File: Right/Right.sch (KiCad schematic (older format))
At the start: 105 parts, among them SW1 SW_PUSH, SW10 SW_PUSH, SW100 SW_Push_Dual_R, SW101 SW_Push_Dual_R, SW102 SW_Push_Dual_R, SW11 SW_PUSH, SW12 SW_PUSH, SW13 SW_PUSH, SW14 SW_PUSH, SW15 SW_PUSH, SW16 SW_PUSH, SW17 SW_PUSH, SW18 SW_PUSH, SW19 SW_PUSH, SW2 SW_PUSH, SW20 SW_PUSH, SW200 SW_SPDT, SW21 SW_PUSH, SW22 SW_PUSH, SW23 SW_PUSH, SW24 SW_PUSH, SW25 SW_PUSH, SW26 SW_PUSH, SW27 SW_PUSH, SW28 SW_PUSH, SW29 SW_PUSH, SW3 SW_PUSH, SW30 SW_PUSH, SW31 SW_PUSH, SW32 SW_PUSH, SW33 SW_PUSH, SW34 SW_PUSH, SW35 SW_PUSH, SW36 SW_PUSH, SW37 SW_PUSH, SW38 SW_PUSH, SW39 SW_PUSH, SW4 SW_PUSH, SW40 SW_PUSH, SW41 SW_PUSH, SW42 SW_PUSH, SW43 SW_PUSH, SW44 SW_PUSH, SW45 SW_PUSH, SW5 SW_PUSH, SW6 SW_PUSH, SW7 SW_PUSH, SW8 SW_PUSH, SW9 SW_PUSH, U1 CH25-2032LF, U2 CH25-2032LF

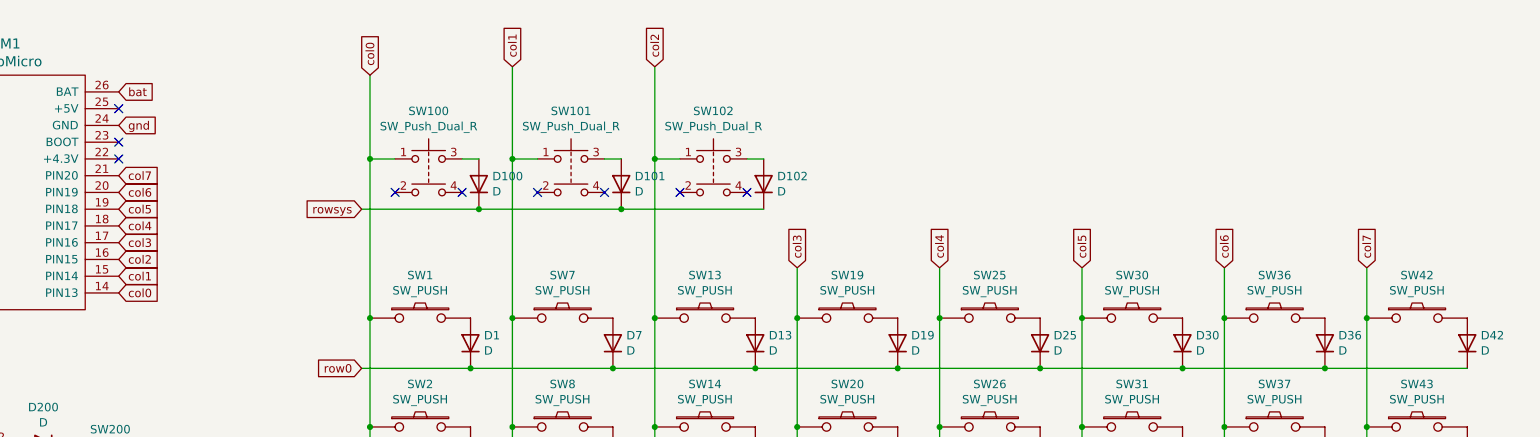
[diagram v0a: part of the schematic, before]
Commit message: 小さく
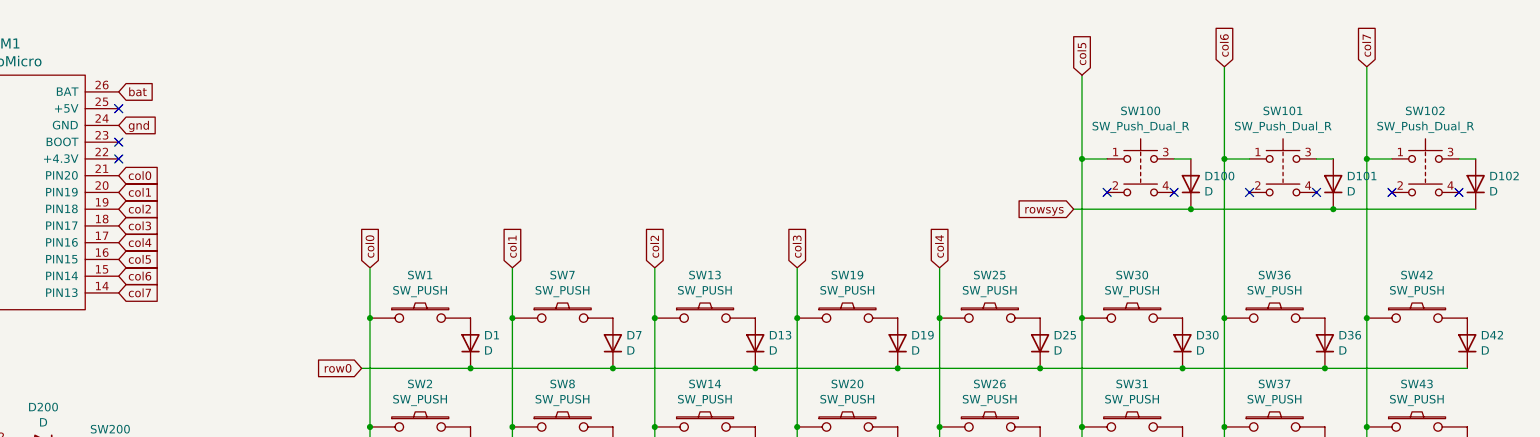
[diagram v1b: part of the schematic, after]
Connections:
- net col0: now also BPM1.21 (PIN20); no longer BPM1.14 (PIN13), SW100.1
- net col1: now also BPM1.20 (PIN19); no longer BPM1.15 (PIN14), SW101.1
- net col2: now also BPM1.19 (PIN18); no longer BPM1.16 (PIN15), SW102.1
- net col3: now also BPM1.18 (PIN17); no longer BPM1.17 (PIN16)
- net col4: now also BPM1.17 (PIN16); no longer BPM1.18 (PIN17)
- net col5: now also BPM1.16 (PIN15), SW100.1; no longer BPM1.19 (PIN18)
- net col6: now also BPM1.15 (PIN14), SW101.1; no longer BPM1.20 (PIN19)
- net col7: now also BPM1.14 (PIN13), SW102.1; no longer BPM1.21 (PIN20)
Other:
- moved on the sheet: D100, D101, D102, SW100, SW101, SW102
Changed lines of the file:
@@
 $EndComp
 Wire Wire Line
-	5750 1200 5750 1750
+	10000 1200 10000 1750
 Connection ~ 5750 2700
 Connection ~ 6350 3000
@@
 	0    -1   -1   0
 $EndComp
-Wire Wire Line
-	8300 2400 8300 2700
 Connection ~ 8300 2700
 Connection ~ 8900 3000
@@
 	0    -1   -1   0
 $EndComp
-Wire Wire Line
-	9150 2400 9150 2700
 Connection ~ 9150 2700
 Connection ~ 9750 3000
@@
 	0    -1   -1   0
 $EndComp
-Wire Wire Line
-	10000 2400 10000 2700
 Connection ~ 10000 2700
 Wire Wire Line
@@
 Text GLabel 4000 6250 0    50   Input ~ 0
 row5
-Text GLabel 4050 1250 1    50   Input ~ 0
+Text GLabel 4050 2400 1    50   Input ~ 0
 col0
-Text GLabel 4900 1200 1    50   Input ~ 0
+Text GLabel 4900 2400 1    50   Input ~ 0
 col1
-Text GLabel 5750 1200 1    50   Input ~ 0
+Text GLabel 5750 2400 1    50   Input ~ 0
 col2
 Text GLabel 6600 2400 1    50   Input ~ 0
@@
 Text GLabel 7450 2400 1    50   Input ~ 0
 col4
-Text GLabel 8300 2400 1    50   Input ~ 0
+Text GLabel 8300 1250 1    50   Input ~ 0
 col5
-Text GLabel 9150 2400 1    50   Input ~ 0
+Text GLabel 9150 1200 1    50   Input ~ 0
 col6
-Text GLabel 10000 2400 1    50   Input ~ 0
+Text GLabel 10000 1200 1    50   Input ~ 0
 col7
 $Comp
@@
 Text GLabel 1150 1850 0    50   Input ~ 0
 row5
-Text GLabel 2550 2550 2    50   Input ~ 0
-col0
-Text GLabel 2550 2450 2    50   Input ~ 0
-col1
-Text GLabel 2550 2350 2    50   Input ~ 0
-col2
-Text GLabel 2550 2250 2    50   Input ~ 0
-col3
-Text GLabel 2550 2150 2    50   Input ~ 0
-col4
-Text GLabel 2550 2050 2    50   Input ~ 0
-col5
-Text GLabel 2550 1950 2    50   Input ~ 0
-col6
-Text GLabel 2550 1850 2    50   Input ~ 0
-col7
 $Comp
 L CH25-2032LF:CH25-2032LF U1
@@
 	1100 3900 1100 3650
 NoConn ~ 2700 3750
-NoConn ~ 4200 1950
-NoConn ~ 4600 1950
+NoConn ~ 8450 1950
+NoConn ~ 8850 1950
 $Comp
 L Device:D D100
 U 1 1 5F386B99
-P 4700 1900
-F 0 "D100" V 4746 1820 50  0000 R CNN
-F 1 "D" V 4655 1820 50  0000 R CNN
-F 2 "Diode_THT:D_DO-35_SOD27_P7.62mm_Horizontal" H 4700 1900 50  0001 C CNN
-F 3 "~" H 4700 1900 50  0001 C CNN
-	1    4700 1900
-	0    -1   -1   0
-$EndComp
-Wire Wire Line
-	4600 1750 4700 1750
-Wire Wire Line
-	4700 2050 4000 2050
-Text GLabel 4000 2050 0    50   Input ~ 0
+P 8950 1900
+F 0 "D100" V 8996 1820 50  0000 R CNN
+F 1 "D" V 8905 1820 50  0000 R CNN
+F 2 "Diode_THT:D_DO-35_SOD27_P7.62mm_Horizontal" H 8950 1900 50  0001 C CNN
+F 3 "~" H 8950 1900 50  0001 C CNN
+	1    8950 1900
+	0    -1   -1   0
+$EndComp
+Wire Wire Line
+	8850 1750 8950 1750
+Wire Wire Line
+	8950 2050 8250 2050
+Text GLabel 8250 2050 0    50   Input ~ 0
 rowsys
 Wire Wire Line
-	4700 2050 5550 2050
-Connection ~ 4700 2050
-Wire Wire Line
-	4050 1250 4050 1750
-Wire Wire Line
-	4200 1750 4050 1750
-Connection ~ 4050 1750
-Wire Wire Line
-	4050 1750 4050 2700
-Wire Wire Line
-	4900 1200 4900 1750
-NoConn ~ 5050 1950
-NoConn ~ 5450 1950
+	8950 2050 9800 2050
+Connection ~ 8950 2050
+Wire Wire Line
+	8300 1250 8300 1750
+Wire Wire Line
+	8450 1750 8300 1750
+Connection ~ 8300 1750
+Wire Wire Line
+	9150 1200 9150 1750
+NoConn ~ 9300 1950
+NoConn ~ 9700 1950
 $Comp
 L Device:D D101
 U 1 1 5F3CEA11
-P 5550 1900
-F 0 "D101" V 5596 1820 50  0000 R CNN
-F 1 "D" V 5505 1820 50  0000 R CNN
-F 2 "Diode_THT:D_DO-35_SOD27_P7.62mm_Horizontal" H 5550 1900 50  0001 C CNN
-F 3 "~" H 5550 1900 50  0001 C CNN
-	1    5550 1900
-	0    -1   -1   0
-$EndComp
-Wire Wire Line
-	5450 1750 5550 1750
-Wire Wire Line
-	5050 1750 4900 1750
-Connection ~ 5550 2050
-Connection ~ 4900 1750
-Wire Wire Line
-	4900 1750 4900 2700
-NoConn ~ 5900 1950
-NoConn ~ 6300 1950
+P 9800 1900
+F 0 "D101" V 9846 1820 50  0000 R CNN
+F 1 "D" V 9755 1820 50  0000 R CNN
+F 2 "Diode_THT:D_DO-35_SOD27_P7.62mm_Horizontal" H 9800 1900 50  0001 C CNN
+F 3 "~" H 9800 1900 50  0001 C CNN
+	1    9800 1900
+	0    -1   -1   0
+$EndComp
+Wire Wire Line
+	9700 1750 9800 1750
+Wire Wire Line
+	9300 1750 9150 1750
+Connection ~ 9800 2050
+Connection ~ 9150 1750
+NoConn ~ 10150 1950
+NoConn ~ 10550 1950
 $Comp
 L Device:D D102
 U 1 1 5F3D4407
-P 6400 1900
-F 0 "D102" V 6446 1820 50  0000 R CNN
-F 1 "D" V 6355 1820 50  0000 R CNN
-F 2 "Diode_THT:D_DO-35_SOD27_P7.62mm_Horizontal" H 6400 1900 50  0001 C CNN
-F 3 "~" H 6400 1900 50  0001 C CNN
-	1    6400 1900
-	0    -1   -1   0
-$EndComp
-Wire Wire Line
-	6300 1750 6400 1750
-Wire Wire Line
-	5900 1750 5750 1750
-Connection ~ 5750 1750
-Wire Wire Line
-	5750 1750 5750 2700
-Wire Wire Line
-	5550 2050 6400 2050
+P 10650 1900
+F 0 "D102" V 10696 1820 50  0000 R CNN
+F 1 "D" V 10605 1820 50  0000 R CNN
+F 2 "Diode_THT:D_DO-35_SOD27_P7.62mm_Horizontal" H 10650 1900 50  0001 C CNN
+F 3 "~" H 10650 1900 50  0001 C CNN
+	1    10650 1900
+	0    -1   -1   0
+$EndComp
+Wire Wire Line
+	10550 1750 10650 1750
+Wire Wire Line
+	10150 1750 10000 1750
+Connection ~ 10000 1750
+Wire Wire Line
+	9800 2050 10650 2050
 Text GLabel 1150 2550 0    50   Input ~ 0
 rowsys
@@
 L My_Library:SW_Push_Dual_R SW102
 U 1 1 5F449060
-P 6100 1750
-F 0 "SW102" H 6100 2035 50  0000 C CNN
-F 1 "SW_Push_Dual_R" H 6100 1944 50  0000 C CNN
-F 2 "Button_Switch_THT:SW_TH_Tactile_Omron_B3F-10xx" H 6100 1950 50  0001 C CNN
-F 3 "" H 6100 1950 50  0001 C CNN
-	1    6100 1750
+P 10350 1750
+F 0 "SW102" H 10350 2035 50  0000 C CNN
+F 1 "SW_Push_Dual_R" H 10350 1944 50  0000 C CNN
+F 2 "Button_Switch_THT:SW_TH_Tactile_Omron_B3F-10xx" H 10350 1950 50  0001 C CNN
+F 3 "" H 10350 1950 50  0001 C CNN
+	1    10350 1750
 	1    0    0    -1
 $EndComp
@@
 L My_Library:SW_Push_Dual_R SW101
 U 1 1 5F44E520
-P 5250 1750
-F 0 "SW101" H 5250 2035 50  0000 C CNN
-F 1 "SW_Push_Dual_R" H 5250 1944 50  0000 C CNN
-F 2 "Button_Switch_THT:SW_TH_Tactile_Omron_B3F-10xx" H 5250 1950 50  0001 C CNN
-F 3 "" H 5250 1950 50  0001 C CNN
-	1    5250 1750
+P 9500 1750
+F 0 "SW101" H 9500 2035 50  0000 C CNN
+F 1 "SW_Push_Dual_R" H 9500 1944 50  0000 C CNN
+F 2 "Button_Switch_THT:SW_TH_Tactile_Omron_B3F-10xx" H 9500 1950 50  0001 C CNN
+F 3 "" H 9500 1950 50  0001 C CNN
+	1    9500 1750
 	1    0    0    -1
 $EndComp
@@
 L My_Library:SW_Push_Dual_R SW100
 U 1 1 5F44F80F
-P 4400 1750
-F 0 "SW100" H 4400 2035 50  0000 C CNN
-F 1 "SW_Push_Dual_R" H 4400 1944 50  0000 C CNN
-F 2 "Button_Switch_THT:SW_TH_Tactile_Omron_B3F-10xx" H 4400 1950 50  0001 C CNN
-F 3 "" H 4400 1950 50  0001 C CNN
-	1    4400 1750
-	1    0    0    -1
-$EndComp
+P 8650 1750
+F 0 "SW100" H 8650 2035 50  0000 C CNN
+F 1 "SW_Push_Dual_R" H 8650 1944 50  0000 C CNN
+F 2 "Button_Switch_THT:SW_TH_Tactile_Omron_B3F-10xx" H 8650 1950 50  0001 C CNN
+F 3 "" H 8650 1950 50  0001 C CNN
+	1    8650 1750
+	1    0    0    -1
+$EndComp
+Wire Wire Line
+	5750 2400 5750 2700
+Wire Wire Line
+	4900 2400 4900 2700
+Wire Wire Line
+	4050 2400 4050 2700
+Wire Wire Line
+	8300 1750 8300 2700
+Wire Wire Line
+	9150 1750 9150 2700
+Wire Wire Line
+	10000 1750 10000 2700
+Text GLabel 2550 2550 2    50   Input ~ 0
+col7
+Text GLabel 2550 2450 2    50   Input ~ 0
+col6
+Text GLabel 2550 2350 2    50   Input ~ 0
+col5
+Text GLabel 2550 2250 2    50   Input ~ 0
+col4
+Text GLabel 2550 2150 2    50   Input ~ 0
+col3
+Text GLabel 2550 2050 2    50   Input ~ 0
+col2
+Text GLabel 2550 1950 2    50   Input ~ 0
+col1
+Text GLabel 2550 1850 2    50   Input ~ 0
+col0
 $EndSCHEMATC

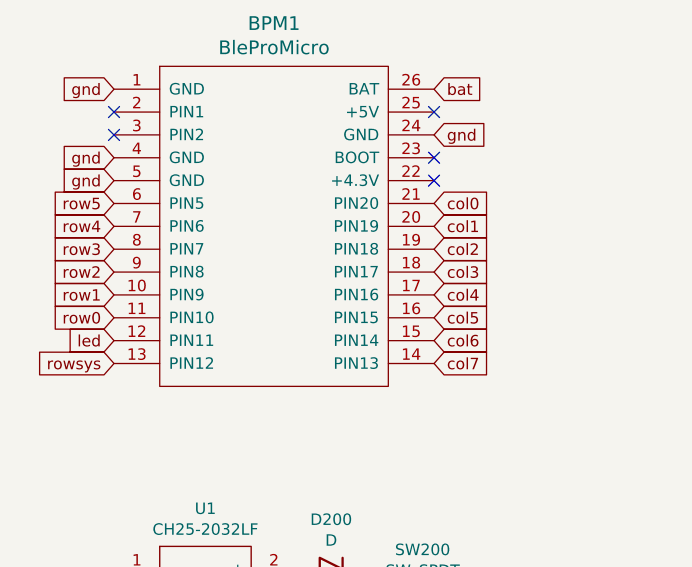
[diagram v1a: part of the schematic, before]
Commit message: 位置調整
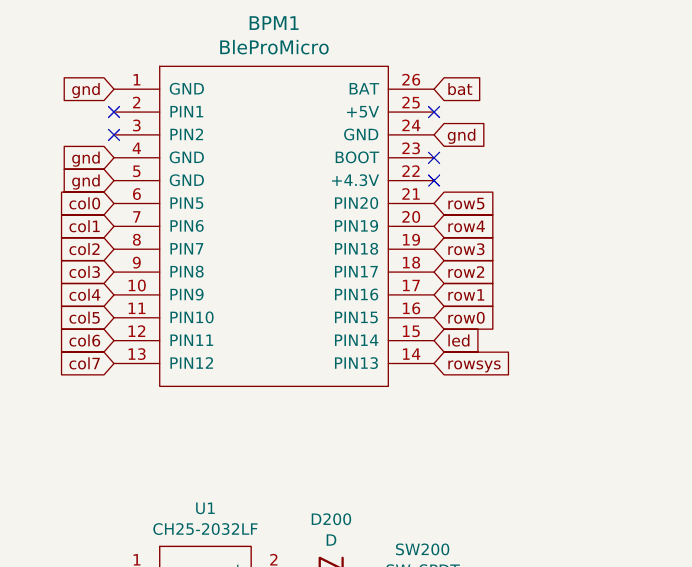
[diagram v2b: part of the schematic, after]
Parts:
- BPM1: footprint mylibrary:BLEMicroPro_reversed -> mylibrary:BLEMicroPro
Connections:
- net col0: now also BPM1.6 (PIN5); no longer BPM1.21 (PIN20)
- net col1: now also BPM1.7 (PIN6); no longer BPM1.20 (PIN19)
- net col2: now also BPM1.8 (PIN7); no longer BPM1.19 (PIN18)
- net col3: now also BPM1.9 (PIN8); no longer BPM1.18 (PIN17)
- net col4: now also BPM1.10 (PIN9); no longer BPM1.17 (PIN16)
- net col5: now also BPM1.11 (PIN10); no longer BPM1.16 (PIN15)
- net col6: now also BPM1.12 (PIN11); no longer BPM1.15 (PIN14)
- net col7: now also BPM1.13 (PIN12); no longer BPM1.14 (PIN13)
- net led: now also BPM1.15 (PIN14); no longer BPM1.12 (PIN11)
- net row0: now also BPM1.16 (PIN15); no longer BPM1.11 (PIN10)
- net row1: now also BPM1.17 (PIN16); no longer BPM1.10 (PIN9)
- net row2: now also BPM1.18 (PIN17); no longer BPM1.9 (PIN8)
- net row3: now also BPM1.19 (PIN18); no longer BPM1.8 (PIN7)
- net row4: now also BPM1.20 (PIN19); no longer BPM1.7 (PIN6)
- net row5: now also BPM1.21 (PIN20); no longer BPM1.6 (PIN5)
- net rowsys: now also BPM1.14 (PIN13); no longer BPM1.13 (PIN12)
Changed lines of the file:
@@
 F 0 "BPM1" H 1850 3337 60  0000 C CNN
 F 1 "BleProMicro" H 1850 3231 60  0000 C CNN
-F 2 "mylibrary:BLEMicroPro_reversed" H 1950 1150 60  0001 C CNN
+F 2 "mylibrary:BLEMicroPro" H 1950 1150 60  0001 C CNN
 F 3 "" H 1950 1150 60  0000 C CNN
 	1    1850 2200
 	1    0    0    -1
 $EndComp
-Text GLabel 1150 2350 0    50   Input ~ 0
+Text GLabel 2550 2350 2    50   Input ~ 0
 row0
-Text GLabel 1150 2250 0    50   Input ~ 0
+Text GLabel 2550 2250 2    50   Input ~ 0
 row1
-Text GLabel 1150 2150 0    50   Input ~ 0
+Text GLabel 2550 2150 2    50   Input ~ 0
 row2
-Text GLabel 1150 2050 0    50   Input ~ 0
+Text GLabel 2550 2050 2    50   Input ~ 0
 row3
-Text GLabel 1150 1950 0    50   Input ~ 0
+Text GLabel 2550 1950 2    50   Input ~ 0
 row4
-Text GLabel 1150 1850 0    50   Input ~ 0
+Text GLabel 2550 1850 2    50   Input ~ 0
 row5
 $Comp
@@
 Text GLabel 1350 5150 0    50   Input ~ 0
 led
-Text GLabel 1150 2450 0    50   Input ~ 0
+Text GLabel 2550 2450 2    50   Input ~ 0
 led
 Wire Wire Line
@@
 Wire Wire Line
 	9800 2050 10650 2050
-Text GLabel 1150 2550 0    50   Input ~ 0
+Text GLabel 2550 2550 2    50   Input ~ 0
 rowsys
 $Comp
@@
 Wire Wire Line
 	10000 1750 10000 2700
-Text GLabel 2550 2550 2    50   Input ~ 0
+Text GLabel 1150 1850 0    50   Input ~ 0
+col0
+Text GLabel 1150 1950 0    50   Input ~ 0
+col1
+Text GLabel 1150 2050 0    50   Input ~ 0
+col2
+Text GLabel 1150 2150 0    50   Input ~ 0
+col3
+Text GLabel 1150 2250 0    50   Input ~ 0
+col4
+Text GLabel 1150 2350 0    50   Input ~ 0
+col5
+Text GLabel 1150 2450 0    50   Input ~ 0
+col6
+Text GLabel 1150 2550 0    50   Input ~ 0
 col7
-Text GLabel 2550 2450 2    50   Input ~ 0
-col6
-Text GLabel 2550 2350 2    50   Input ~ 0
-col5
-Text GLabel 2550 2250 2    50   Input ~ 0
-col4
-Text GLabel 2550 2150 2    50   Input ~ 0
-col3
-Text GLabel 2550 2050 2    50   Input ~ 0
-col2
-Text GLabel 2550 1950 2    50   Input ~ 0
-col1
-Text GLabel 2550 1850 2    50   Input ~ 0
-col0
 $EndSCHEMATC
